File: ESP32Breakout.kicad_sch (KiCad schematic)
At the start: 3 parts, among them U1 ESP32-S3

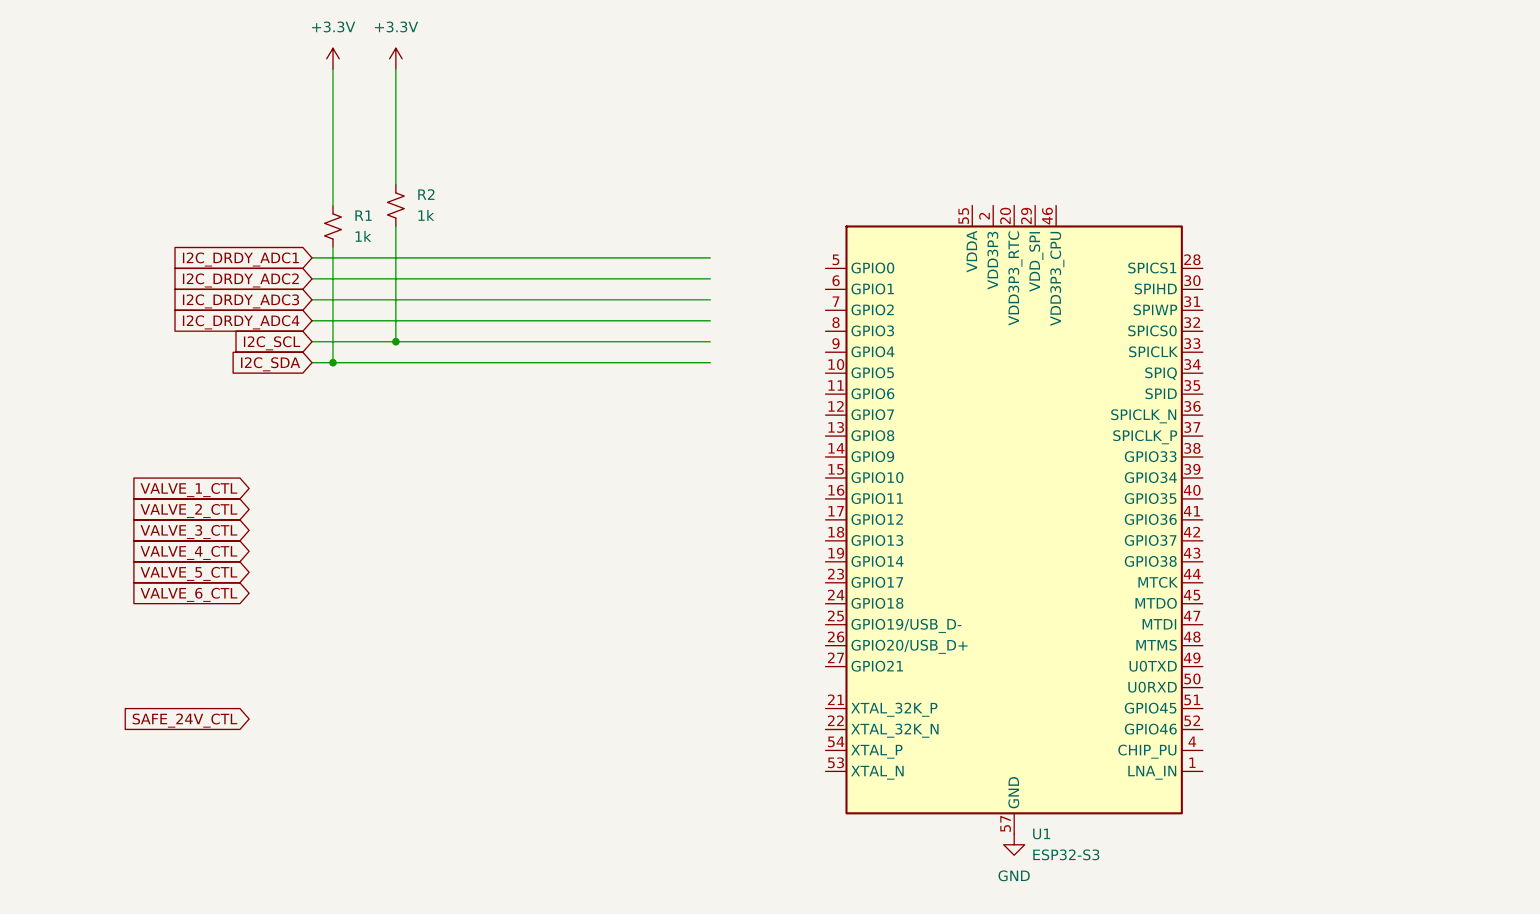
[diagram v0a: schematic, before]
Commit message: v0.1 sch. Add devkit c1 footprint
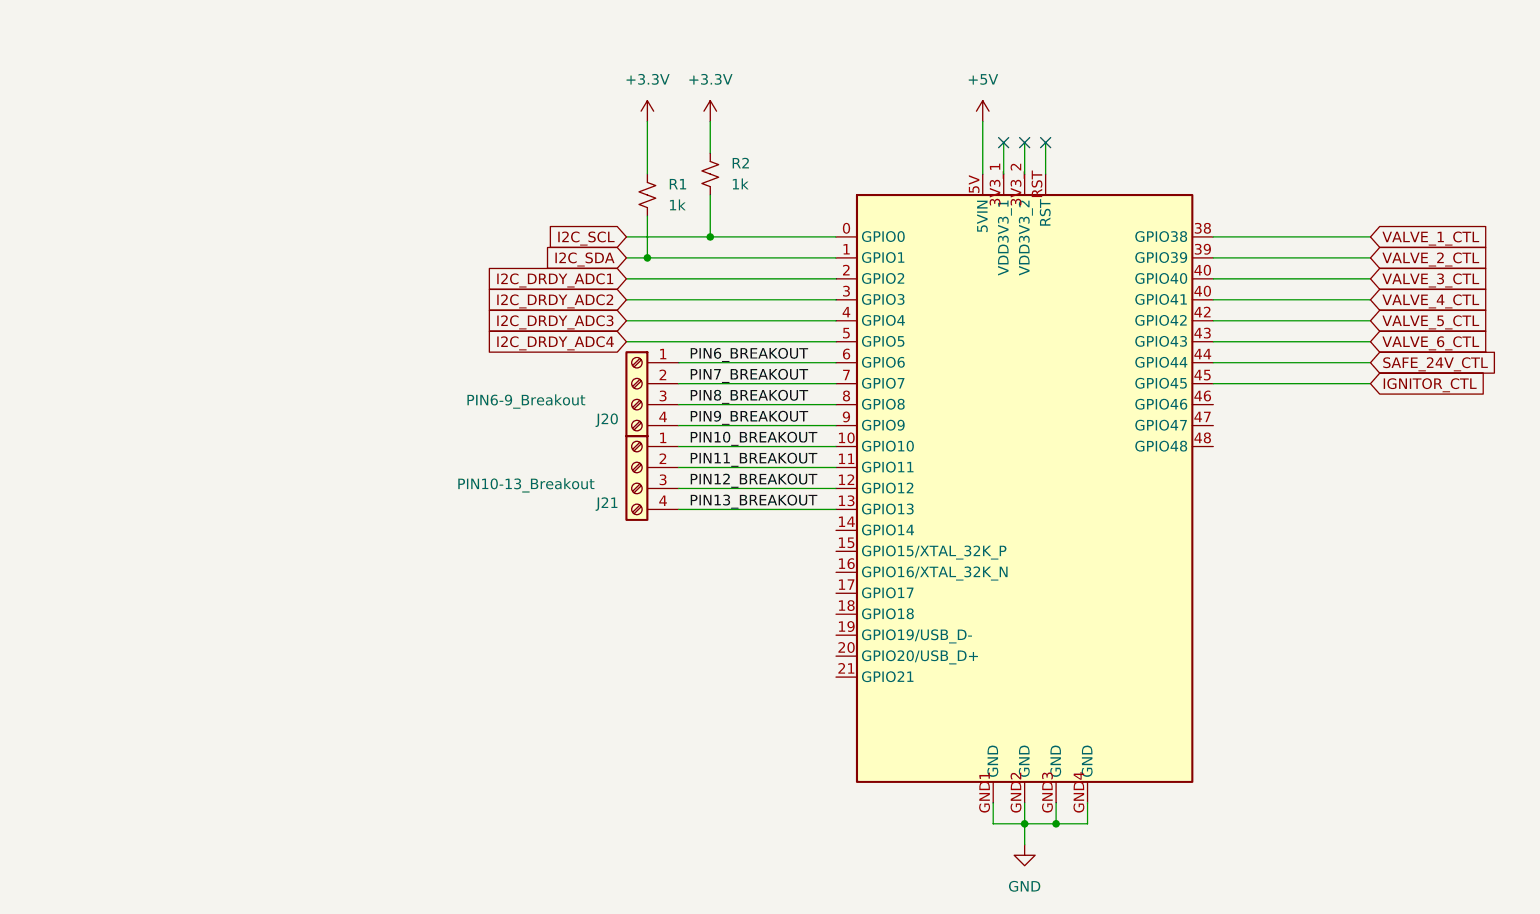
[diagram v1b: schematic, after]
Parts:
- removed U1: ESP32-S3, Package_DFN_QFN:QFN-56-1EP_7x7mm_P0.4mm_EP4x4mm, symbol MCU_Espressif:ESP32-S3
- added J20: PIN6-9_Breakout, TerminalBlock:TerminalBlock_Xinya_XY308-2.54-4P_1x04_P2.54mm_Horizontal, symbol Connector:Screw_Terminal_01x04
- added J21: PIN10-13_Breakout, TerminalBlock:TerminalBlock_Xinya_XY308-2.54-4P_1x04_P2.54mm_Horizontal, symbol Connector:Screw_Terminal_01x04
- added U1: ESP32-S3, Library:ESP32_Devkit_C1_Noah, symbol ESP32_Devkit_C1_Noah:ESP32-S3
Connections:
- net GND: now also U1.GND1 (GND), U1.GND2 (GND), U1.GND3 (GND), U1.GND4 (GND)
- net I2C_DRDY_ADC1: now also U1.2 (GPIO2)
- net I2C_DRDY_ADC2: now also U1.3 (GPIO3)
- net I2C_DRDY_ADC3: now also U1.4 (GPIO4)
- net I2C_DRDY_ADC4: now also U1.5 (GPIO5)
- net I2C_SCL: now also U1.0 (GPIO0)
- net I2C_SDA: now also U1.1 (GPIO1)
- net SAFE_24V_CTL: now also U1.44 (GPIO44)
- net VALVE_1_CTL: now also U1.38 (GPIO38)
- net VALVE_2_CTL: now also U1.39 (GPIO39)
- net VALVE_3_CTL: now also U1.40 (GPIO41)
- net VALVE_4_CTL: now also U1.40 (GPIO41)
- net VALVE_5_CTL: now also U1.42 (GPIO42)
- net VALVE_6_CTL: now also U1.43 (GPIO43)
- new net +5V: U1.5V (5VIN)
- new net IGNITOR_CTL: U1.45 (GPIO45)
- new net PIN10_BREAKOUT: J21.1 (Pin_1), U1.10 (GPIO10)
- new net PIN11_BREAKOUT: J21.2 (Pin_2), U1.11 (GPIO11)
- new net PIN12_BREAKOUT: J21.3 (Pin_3), U1.12 (GPIO12)
- new net PIN13_BREAKOUT: J21.4 (Pin_4), U1.13 (GPIO13)
- new net PIN6_BREAKOUT: J20.1 (Pin_1), U1.6 (GPIO6)
- new net PIN7_BREAKOUT: J20.2 (Pin_2), U1.7 (GPIO7)
- new net PIN8_BREAKOUT: J20.3 (Pin_3), U1.8 (GPIO8)
- new net PIN9_BREAKOUT: J20.4 (Pin_4), U1.9 (GPIO9)
- no-connect marks 0 -> 3
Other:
- moved on the sheet: R1, R2

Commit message: Almost done routing
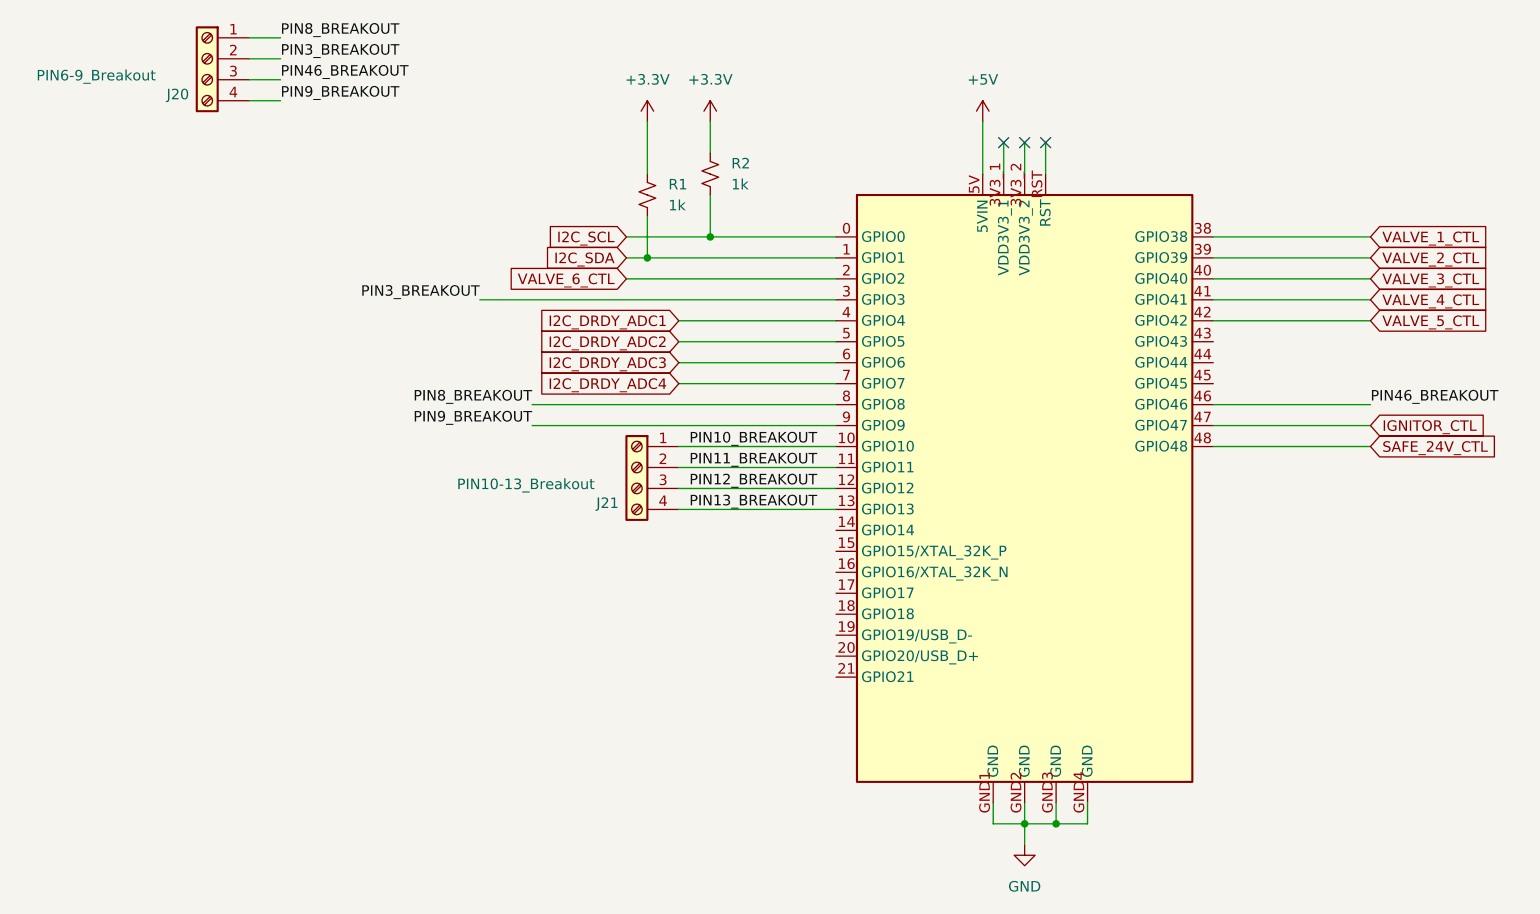
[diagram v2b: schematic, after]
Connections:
- net I2C_DRDY_ADC1: now also U1.4 (GPIO4); no longer U1.2 (GPIO2)
- net I2C_DRDY_ADC2: now also U1.5 (GPIO5); no longer U1.3 (GPIO3)
- net I2C_DRDY_ADC3: now also U1.6 (GPIO6); no longer U1.4 (GPIO4)
- net I2C_DRDY_ADC4: now also U1.7 (GPIO7); no longer U1.5 (GPIO5)
- net IGNITOR_CTL: now also U1.47 (GPIO47); no longer U1.45 (GPIO45)
- net PIN8_BREAKOUT: now also J20.1 (Pin_1); no longer J20.3 (Pin_3)
- net SAFE_24V_CTL: now also U1.48 (GPIO48); no longer U1.44 (GPIO44)
- net VALVE_4_CTL: now also U1.41 (GPIO41); no longer U1.40 (GPIO41)
- net VALVE_6_CTL: now also U1.2 (GPIO2); no longer U1.43 (GPIO43)
- net PIN46_BREAKOUT: now reaches U1.46 (GPIO46)
- net PIN46_BREAKOUT: now also J20.3 (Pin_3)
- removed net PIN6_BREAKOUT: J20.1 (Pin_1), U1.6 (GPIO6)
- net PIN7_BREAKOUT renamed PIN3_BREAKOUT
- net PIN3_BREAKOUT: now also U1.3 (GPIO3); no longer U1.7 (GPIO7)
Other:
- moved on the sheet: J20
